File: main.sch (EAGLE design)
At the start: 36 parts, among them IC1 ATTINY13A-SSH, IC2 TP4056-42-ESOP8, IC3 LM27313XMFX_NOPB, T1A 2N4401, T1B NPN, X1 MINI-USB-UX60A-MB-5ST

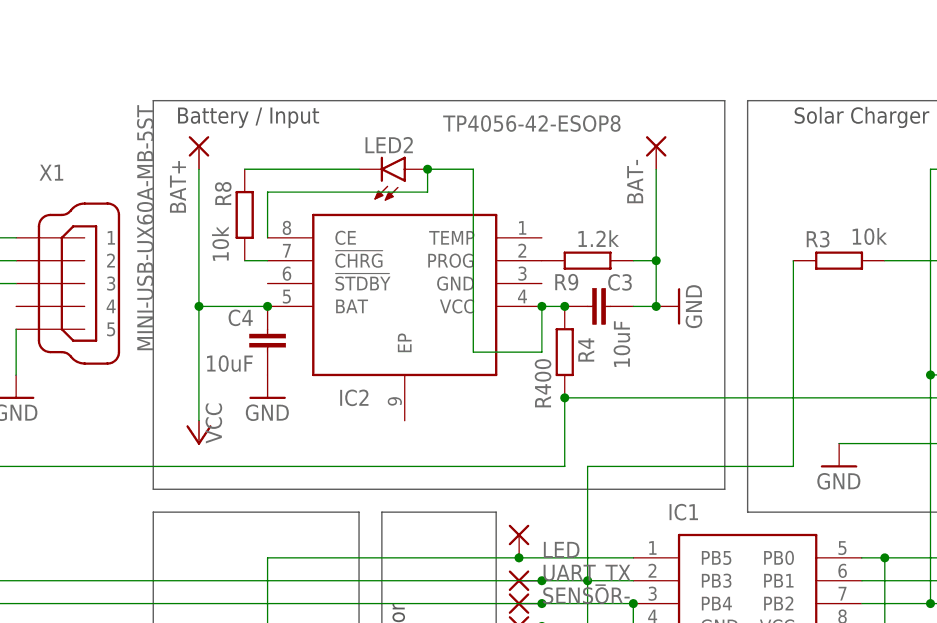
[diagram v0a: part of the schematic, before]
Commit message: new graphics
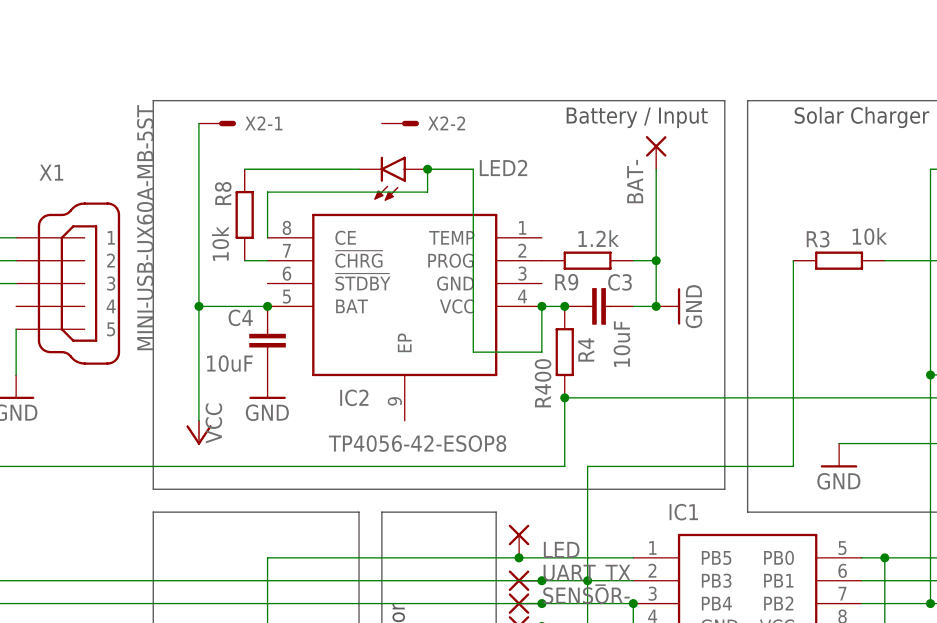
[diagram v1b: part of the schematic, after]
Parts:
- removed BAT+: (no value), wirepad:1,6/0,9
- added X2: 332-02, con-garry:332-02
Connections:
- net VCC: now also X2-1.S; no longer BAT+.P
